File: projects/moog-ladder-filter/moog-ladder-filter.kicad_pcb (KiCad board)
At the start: 2 copper layers, 59.6 x 106 mm, 42 parts, among them J1 02x05_Eurorack_power, J2 IN1, J3 IN2, J4 CV_IN_FREQ, J5 IN2, Q1 MMDT3904, U1 SSI2144, U2 TL072

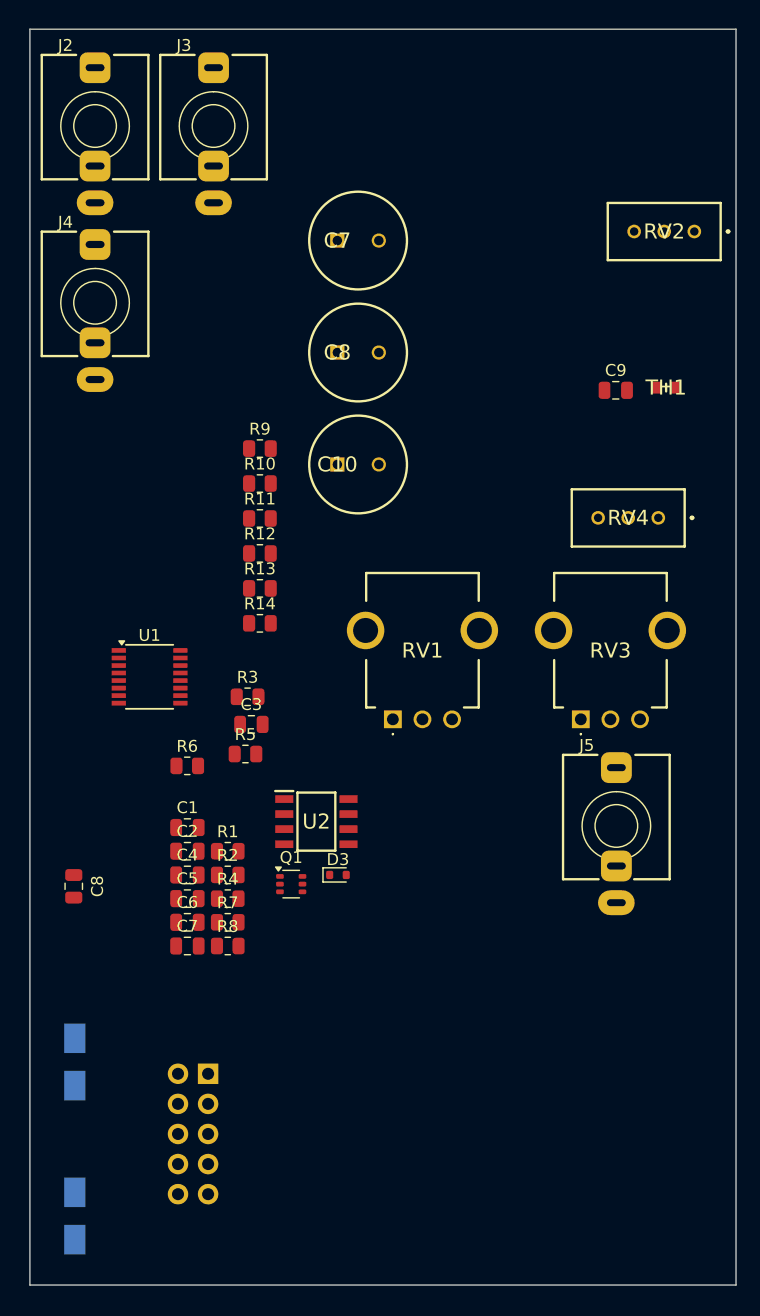
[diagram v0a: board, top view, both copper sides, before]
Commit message: update routing using AI
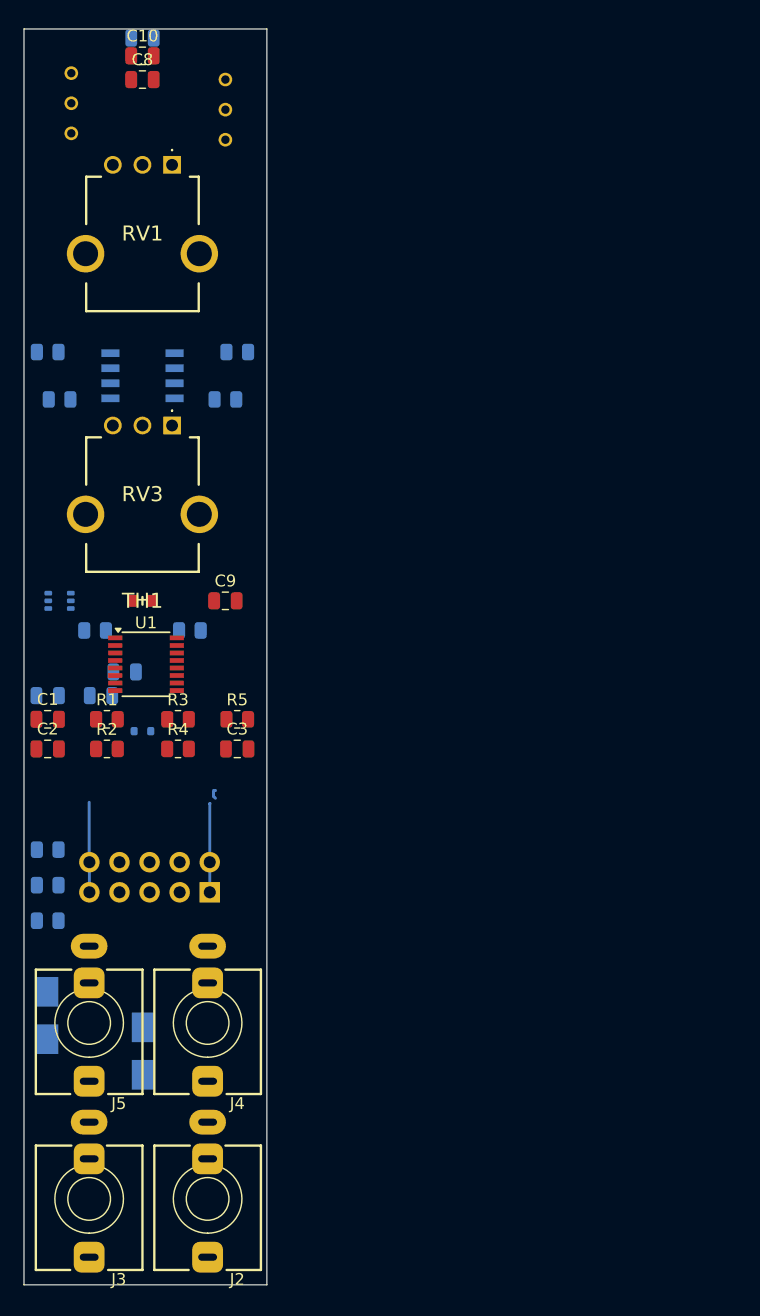
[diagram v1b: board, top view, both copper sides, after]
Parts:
- removed the C7 at (124.5, 65.6)
- removed the C8 at (124.5, 75.0)
- removed the C8 at (102.2, 120.1)
- added C8: 10u, Capacitor_SMD:C_0805_2012Metric, F.Cu at (108.0, 52.0)
- C10: footprint Eurorack:CAPPRD350W60D825H1300 -> Capacitor_SMD:C_0805_2012Metric
- C4, C5, C6, D3, Q1, R10, R11, R12, R13, R14, R6, R7, R8, R9, RV2, RV4, U2: moved to B.Cu
- C7: value 10n -> 10u; moved to B.Cu
- moved J3 91.2 mm to (103.5, 146.5), turned to 180 degrees
- moved J2 91.1 mm to (113.5, 146.5), turned to 180 degrees
- moved C7 76.7 mm to (108.0, 48.5), turned to 180 degrees
- moved J4 61.5 mm to (113.5, 131.6), turned to 180 degrees
- moved RV2 53.2 mm to (102.0, 56.5), turned to -90 degrees
- moved R8 52.4 mm to (100.0, 75.0), turned to 180 degrees
- moved RV1 50.4 mm to (110.5, 59.2), turned to 180 degrees
- moved RV4 48.5 mm to (115.0, 57.1), turned to -90 degrees
- moved TH1 47.7 mm to (108.0, 96.0)
- moved J5 47.5 mm to (103.5, 131.6), turned to 180 degrees
- moved RV3 42.5 mm to (110.5, 81.2), turned to 180 degrees
- moved U2 40.4 mm to (108.0, 77.0), turned to 180 degrees
- moved C10 38.2 mm to (108.0, 50.0)
- moved C9 37.4 mm to (115.0, 96.0)
- moved Q1 30.9 mm to (101.0, 96.0), turned to 180 degrees
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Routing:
- net Net-(D2-K): track 0.00 -> 8.25 mm
- net Net-(D1-A): track 0.00 -> 7.61 mm
- added copper zone on In1.Cu, net GND
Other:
- board size 59.6 x 106 mm -> 20.5 x 106 mm
- copper layers 2 -> 4
